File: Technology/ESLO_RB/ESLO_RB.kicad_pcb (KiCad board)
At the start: 4 copper layers, 27 x 13 mm, 65 parts, among them CN3 1000pF, CN4 1uF, CN7 1000pF, CN8 1uF, CN9 4700pF, J1 Board to Board, J2 Conn_01x10_Female, U1 TPS62740, U10 MT29F2G01ABBGDWB-IT:G TR, U2 LP5907MFX-1.5, U3 CC2652RB, U4 2450BM14G0011, U5 MAX1720, U6 TPS72301DDCT, U7 ADS1294, U8 LSM303AGR, U9 CY15V104QI-20LPXC

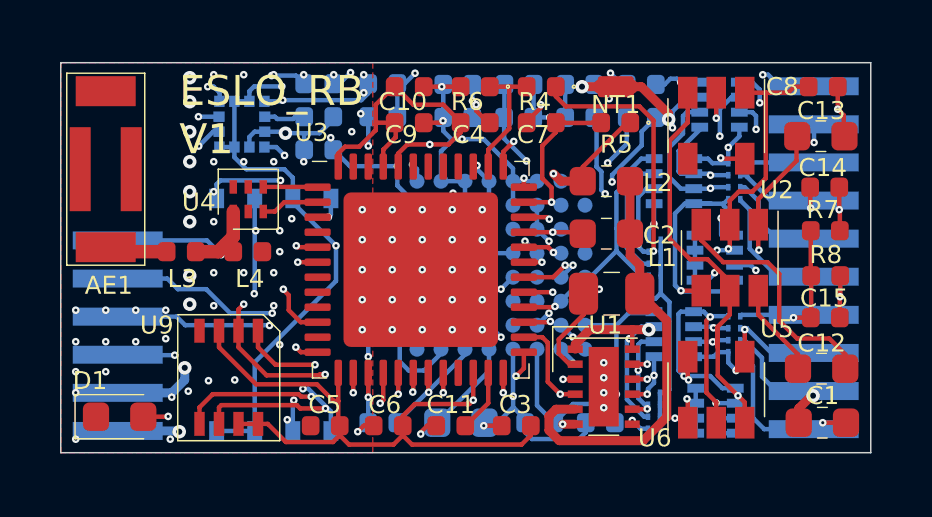
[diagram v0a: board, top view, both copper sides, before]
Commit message: Submit ESLO_RB for mfg w PCBONLINE
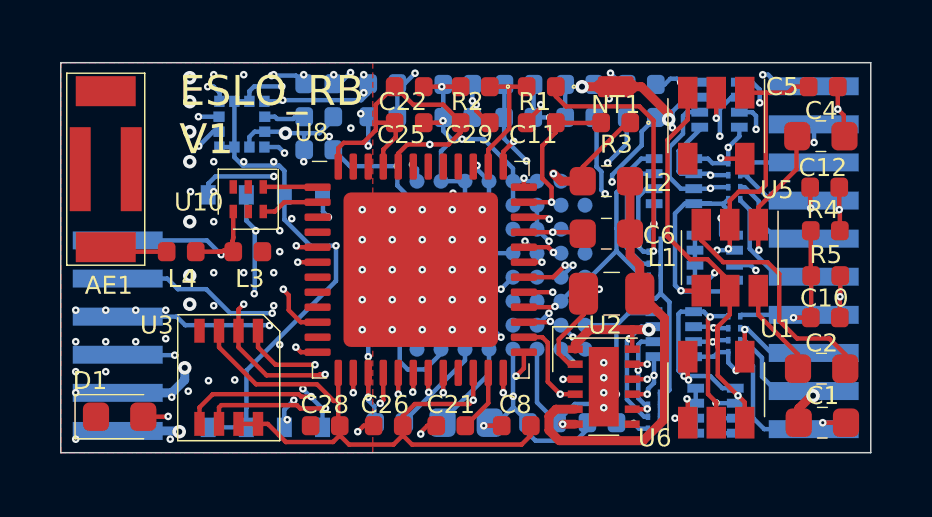
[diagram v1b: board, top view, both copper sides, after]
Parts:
- removed the C20 at (140.5, 101.7)
- removed the C21 at (142.5, 101.7)
- removed C31: 22uF, Capacitor_SMD:C_0603_1608Metric
- removed C32: 1uF, Capacitor_SMD:C_0402_1005Metric
- removed the R6 at (138.3, 90.5)
- added C13: 22uF, Capacitor_SMD:C_0603_1608Metric, B.Cu at (138.0, 101.7)
- added C14: 1uF, Capacitor_SMD:C_0402_1005Metric, B.Cu at (135.5, 101.7)
- added C24: 1uF, Capacitor_SMD:C_0402_1005Metric, B.Cu at (140.6, 101.7)
- added C27: 0.1uF, Capacitor_SMD:C_0402_1005Metric, B.Cu at (142.5, 101.7)
- added R2: 100k, LED_SMD:LED_0402_1005Metric, F.Cu at (138.3, 90.5)
- C11: renamed from C7; value 100nF -> 0.1uF
- C22: renamed from C10; value 100nF -> 0.1uF
- C25: renamed from C9; value 100nF -> 0.1uF
- C26: renamed from C6; value 100nF -> 0.1uF
- C28: renamed from C5; value 100nF -> 0.1uF
- C29: renamed from C4; value 100nF -> 0.1uF
- C7: renamed from C30; value 220nF -> 0.22uF
- J1: renamed from J2; value Conn_01x10_Female -> 10POS Biopotentials
- J2: renamed from J1; value Board to Board -> 6POS Power/JTAG
- moved U7 0.30 mm to (131.3, 98.0)
- renumbered C15 to C10, C14 to C12, C33 to C15, C34 to C16, C35 to C18, C36 to C19, C12 to C2, C19 to C20, C11 to C21, C29 to C23, C26 to C3, C13 to C4, C8 to C5, C2 to C6, C3 to C8, C16 to C9, CN9 to CN1, CN3 to CN2, CN7 to CN3, CN8 to CN5, L4 to L3, L3 to L4, R4 to R1, R5 to R3, R7 to R4, R8 to R5, R2 to R6, R3 to R7, R11 to R8, RN5 to RN2, RN2 to RN3, RN6 to RN4, U5 to U1, U4 to U10, U1 to U2, U9 to U3, U8 to U4, U2 to U5, U10 to U7, U3 to U8, U7 to U9
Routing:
- net VDD: track 90.6 -> 91.2 mm
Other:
- rule trace_min: 0.15 -> 0.12
